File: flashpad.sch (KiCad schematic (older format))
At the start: 23 parts, among them SW1 BOOT, SW2 RESET, U1 ATmega328P-PU, U2 ATmega32A-PU

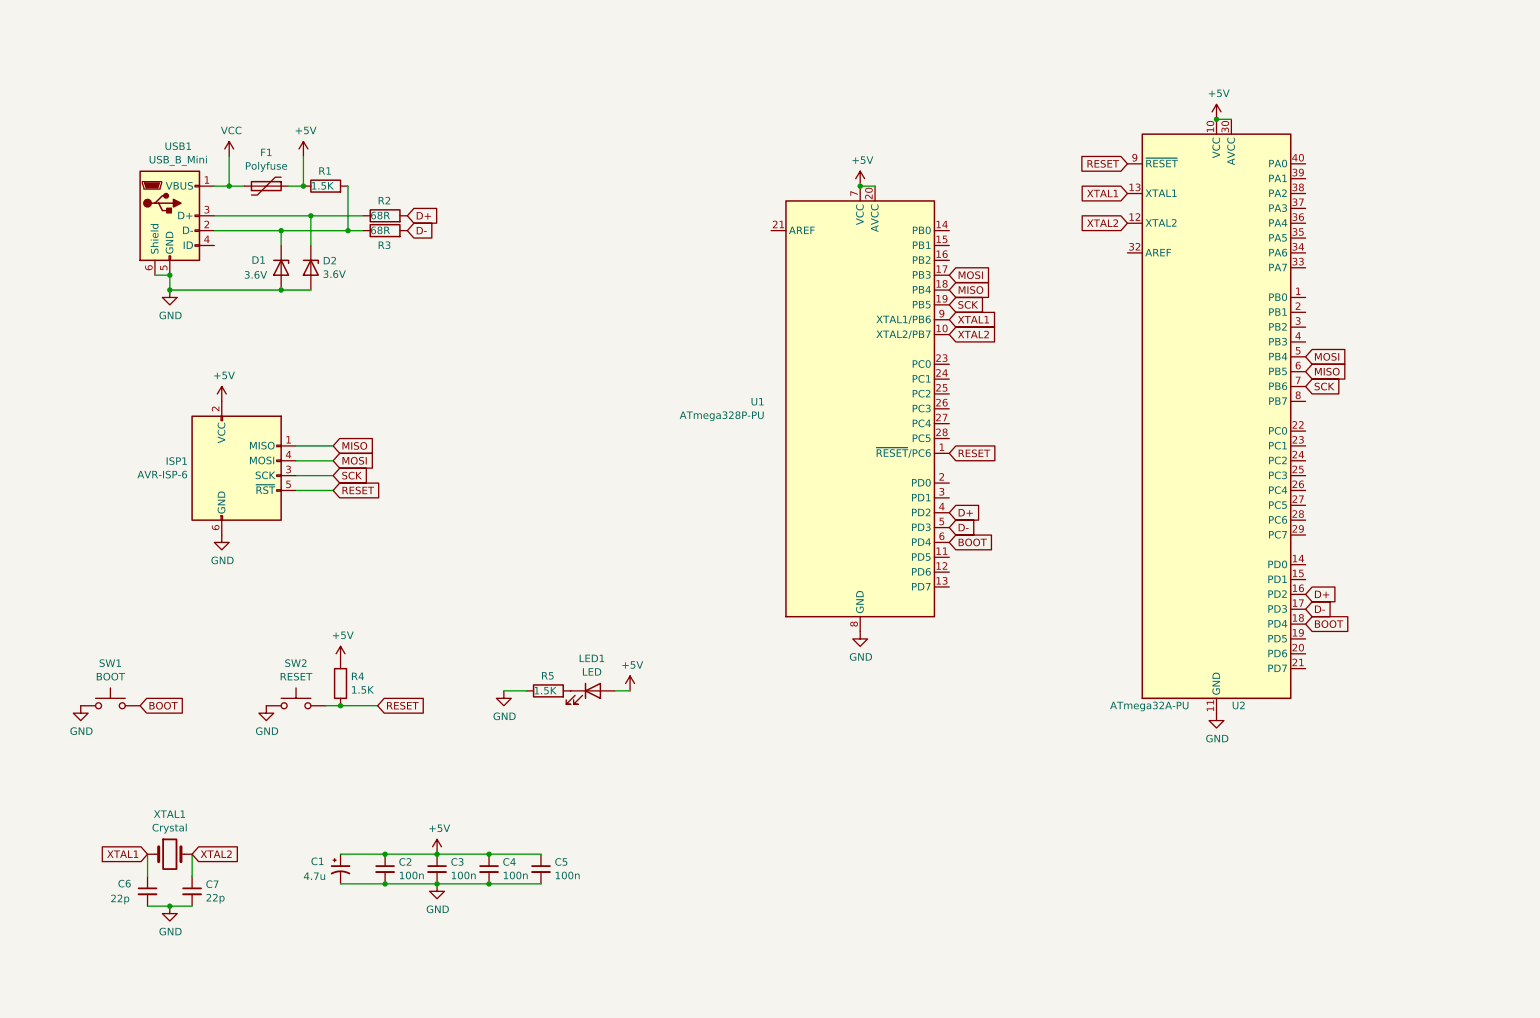
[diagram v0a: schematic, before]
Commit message: rev2
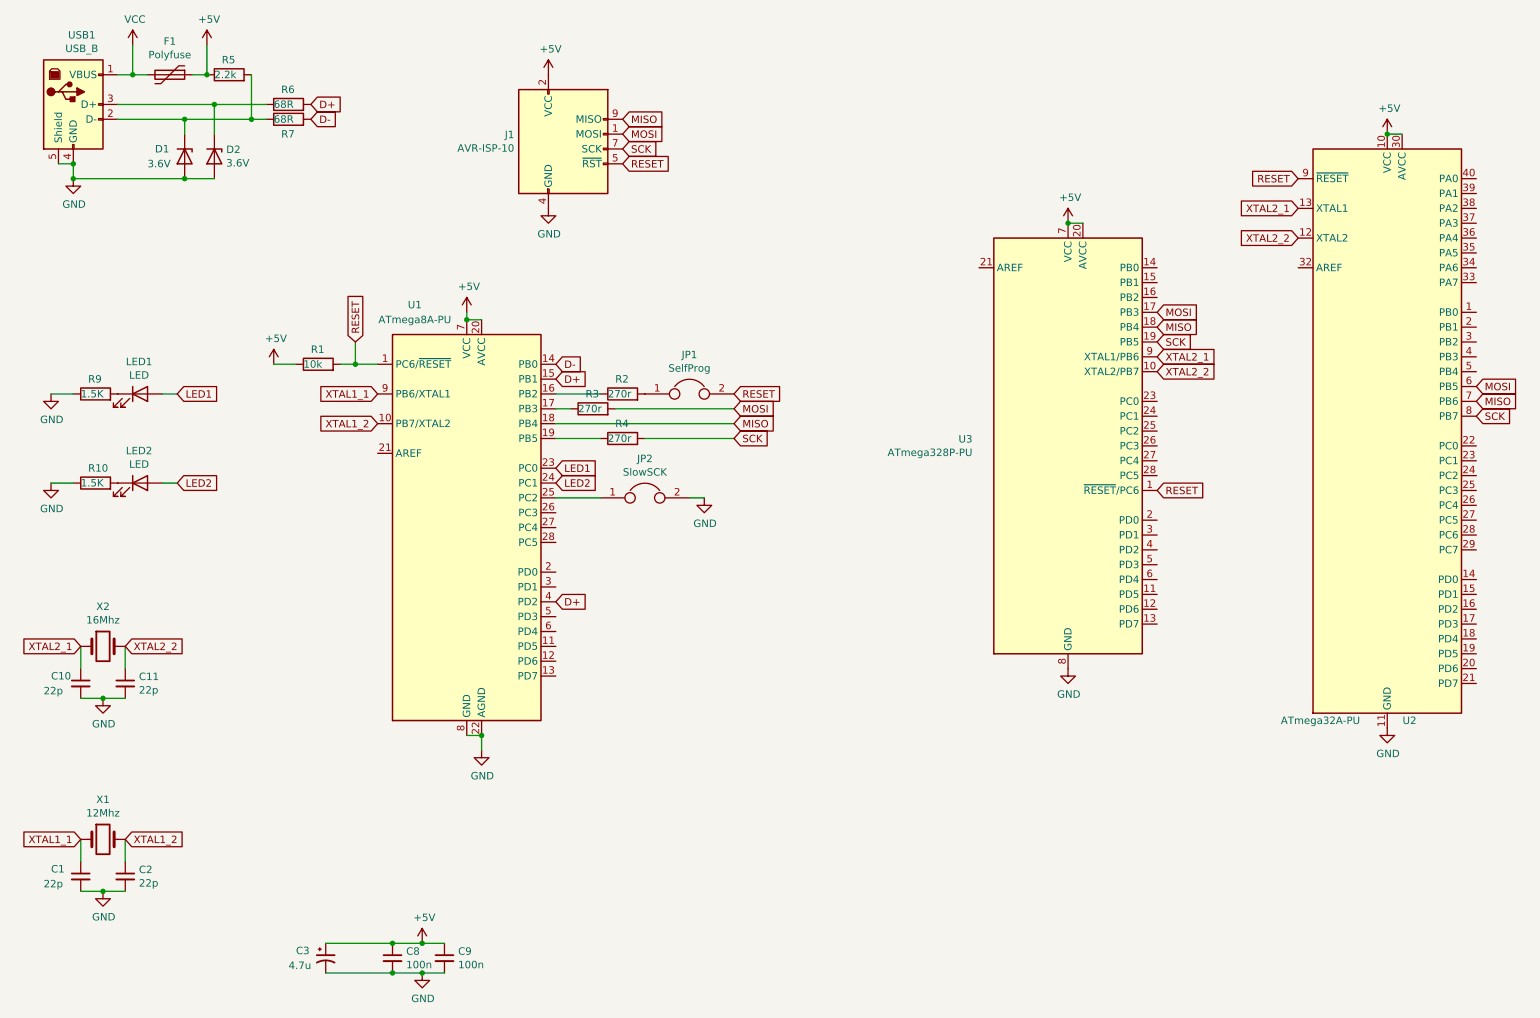
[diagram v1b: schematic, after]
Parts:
- removed C3, C4, C5: 100n, Capacitor_THT:C_Disc_D5.0mm_W2.5mm_P2.50mm, symbol Device:C_Small
- removed ISP1: AVR-ISP-6, Connector_PinHeader_2.54mm:PinHeader_2x03_P2.54mm_Horizontal, symbol Connector:AVR-ISP-6
- removed R5: 1.5K, Resistor_THT:R_Axial_DIN0204_L3.6mm_D1.6mm_P7.62mm_Horizontal, symbol Device:R
- removed SW1: BOOT, Button_Switch_THT:SW_PUSH_6mm, symbol Switch:SW_Push
- removed SW2: RESET, Button_Switch_THT:SW_PUSH_6mm, symbol Switch:SW_Push
- removed USB1: USB_B_Mini, custom_parts:USB_Mini, symbol Connector:USB_B_Mini
- added C1: 22p, Capacitor_THT:C_Disc_D5.0mm_W2.5mm_P5.00mm, symbol Device:C_Small
- added C8, C9: 100n, Capacitor_THT:C_Disc_D5.0mm_W2.5mm_P2.50mm, symbol Device:C_Small
- added J1: AVR-ISP-10, Connector_PinHeader_2.54mm:PinHeader_2x05_P2.54mm_Vertical, symbol Connector:AVR-ISP-10
- added JP1: SelfProg, Connector_PinHeader_2.54mm:PinHeader_1x02_P2.54mm_Vertical, symbol Device:Jumper
- added JP2: SlowSCK, Connector_PinHeader_2.54mm:PinHeader_1x02_P2.54mm_Vertical, symbol Device:Jumper
- added LED2: LED, LED_THT:LED_D5.0mm, symbol Device:LED
- added R1: 10k, Resistor_THT:R_Axial_DIN0204_L3.6mm_D1.6mm_P7.62mm_Horizontal, symbol Device:R
- added R10, R9: 1.5K, Resistor_THT:R_Axial_DIN0204_L3.6mm_D1.6mm_P7.62mm_Horizontal, symbol Device:R
- added R2, R3: 270r, Resistor_THT:R_Axial_DIN0204_L3.6mm_D1.6mm_P7.62mm_Horizontal, symbol Device:R
- added U1: ATmega8A-PU, Package_DIP:DIP-28_W7.62mm, symbol MCU_Microchip_ATmega:ATmega8A-PU
- added USB1: USB_B, Connector_USB:USB_B_OST_USB-B1HSxx_Horizontal, symbol Connector:USB_B
- added X1: 12Mhz, Crystal:Crystal_HC49-4H_Vertical, symbol Device:Crystal
- C2: value 100n -> 22p; footprint Capacitor_THT:C_Disc_D5.0mm_W2.5mm_P2.50mm -> Capacitor_THT:C_Disc_D5.0mm_W2.5mm_P5.00mm
- LED1: footprint LED_THT:LED_D3.0mm -> LED_THT:LED_D5.0mm
- R4: value 1.5K -> 270r
- R5: renamed from R1; value 1.5K -> 2.2k
- U2: footprint Package_DIP:DIP-40_W15.24mm_Socket -> Socket:DIP_Socket-40_W11.9_W12.7_W15.24_W17.78_W18.5_3M_240-1280-00-0602J
- U3: renamed from U1; footprint Package_DIP:DIP-28_W7.62mm_Socket -> custom_parts:DIP_Socket-28_flipped
- X2: renamed from XTAL1; value Crystal -> 16Mhz
- renumbered C6 to C10, C7 to C11, C1 to C3, R2 to R6, R3 to R7
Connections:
- net +5V: now also C8.1, C9.1, J1.2 (VCC), R1.1, U1.20 (AVCC), U1.7 (VCC); no longer C2.1, LED1.2 (A), R4.2
- net D+: now also U1.15 (PB1), U1.4 (PD2); no longer U2.16 (PD2), U3.4 (PD2)
- net D-: now also U1.14 (PB0); no longer U2.17 (PD3), U3.5 (PD3)
- net GND: now also C1.2, C8.2, C9.2, J1.10 (GND), J1.4 (GND), J1.6 (GND), J1.8 (GND), JP2.2, R10.1, R9.1, U1.22 (AGND), U1.8 (GND), USB1.4 (GND), USB1.5 (Shield)
- net MISO: now also U2.7 (PB6), J1.9 (MISO), U1.18 (PB4); no longer U2.6 (PB5)
- net MOSI: now also U2.6 (PB5), J1.1 (MOSI), R3.2; no longer U2.5 (PB4)
- net RESET: now also J1.5 (~RST), JP1.2, R1.2, U1.1 (PC6/~RESET); no longer R4.1
- net SCK: now also R4.2, U2.8 (PB7), J1.7 (SCK); no longer U2.7 (PB6)
- net VCC: now also USB1.1 (VBUS)
- net at D1.1 (K), R5.2, R7.1: now also USB1.2 (D-)
- net at D2.1 (K), R6.1: now also USB1.3 (D+)
- net at LED1.1 (K): now also R9.2
- net BOOT: no longer names the net of U3.6 (PD4)
- net BOOT: no longer U2.18 (PD4)
- net XTAL1 renamed XTAL2_1
- net XTAL2 renamed XTAL2_2
- new net: JP2.1, U1.25 (PC2)
- new net: JP1.1, R2.2
- new net: R2.1, U1.16 (PB2)
- new net: R3.1, U1.17 (PB3)
- new net: R4.1, U1.19 (PB5)
- new net: LED2.1 (K), R10.2
- new net LED1: LED1.2 (A), U1.23 (PC0)
- new net LED2: LED2.2 (A), U1.24 (PC1)
- new net XTAL1_1: C1.1, U1.9 (PB6/XTAL1), X1.1
- new net XTAL1_2: C2.1, U1.10 (PB7/XTAL2), X1.2
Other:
- moved on the sheet: C10, C11, C3, D1, D2, F1, R5, R6, R7, U2, U3, X2
